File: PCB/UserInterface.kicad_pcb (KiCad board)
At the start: 2 copper layers, 8 parts, among them J10 B2B-PH-K-S, J11 B2B-PH-K-S, J2 Conn_01x12, J3 Conn_01x16, J9 B3B-PH-K-S

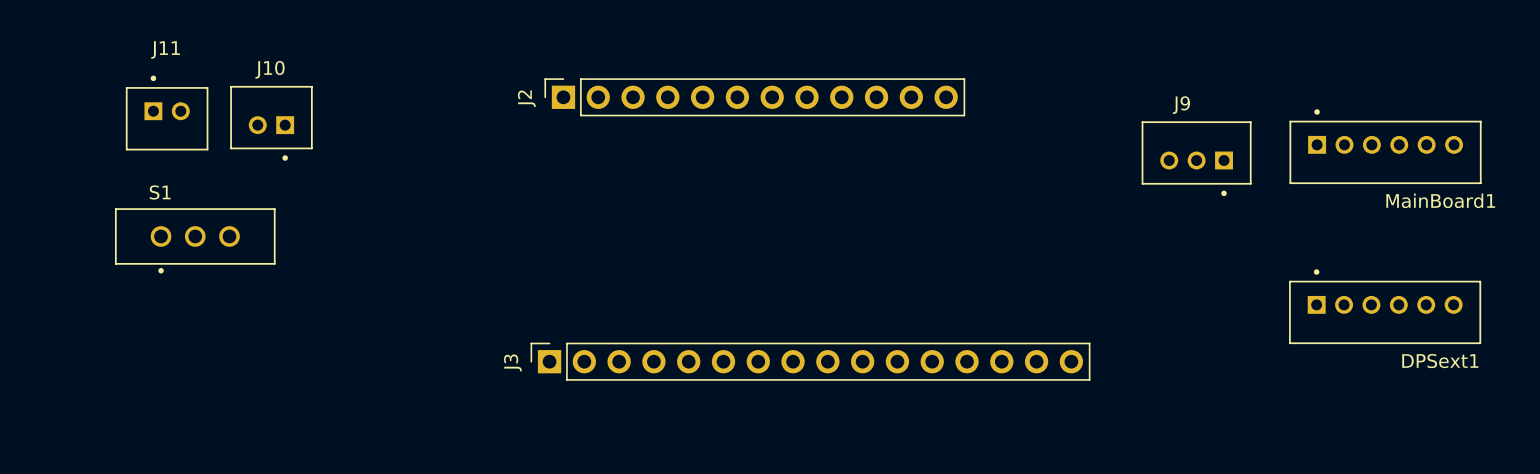
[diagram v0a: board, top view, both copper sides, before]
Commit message: Add files via upload
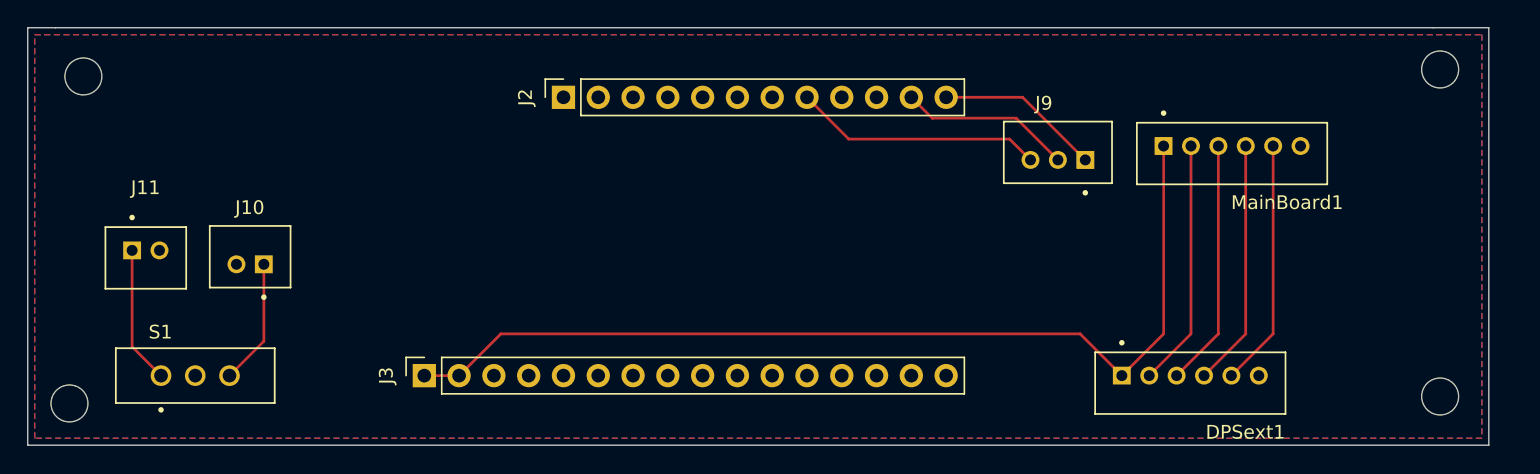
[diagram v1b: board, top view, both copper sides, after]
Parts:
- added REF**: MountingHole_2.7mm_M2.5_ISO7380, MountingHole:MountingHole_2.7mm_M2.5_ISO7380, F.Cu at (73.7, 139.2)
- added REF**: MountingHole_2.7mm_M2.5_ISO7380, MountingHole:MountingHole_2.7mm_M2.5_ISO7380, F.Cu at (173.7, 138.7)
- added REF**: MountingHole_2.7mm_M2.5_ISO7380, MountingHole:MountingHole_2.7mm_M2.5_ISO7380, F.Cu at (173.7, 114.8)
- added REF**: MountingHole_2.7mm_M2.5_ISO7380, MountingHole:MountingHole_2.7mm_M2.5_ISO7380, F.Cu at (74.7, 115.3)
- moved DPSext1 15.1 mm to (155.5, 137.7)
- moved MainBoard1 11.2 mm to (158.5, 120.9)
- moved J10 10.3 mm to (86.9, 128.5)
- moved J11 10.3 mm to (79.2, 128.6)
- moved S1 10.2 mm to (82.8, 137.2)
- moved J9 10.1 mm to (145.8, 120.9)
- moved J3 9.20 mm to (99.6, 137.2)
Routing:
- net /3V3: track 0.00 -> 71.5 mm
- net /OLEDBUTA: track 0.00 -> 18.2 mm
- net /DPSMOSI: track 0.00 -> 18.0 mm
- net /DPSMISO: track 0.00 -> 18.0 mm
- net /DPSCLK: track 0.00 -> 18.0 mm
- net /CS2: track 0.00 -> 18.0 mm
- net /OLEDSCL: track 0.00 -> 12.6 mm
- net /OLEDSDA: track 0.00 -> 12.1 mm
- net Net-(J11-Pad1): track 0.00 -> 10.0 mm
- net Net-(J10-Pad1): track 0.00 -> 9.17 mm
- added copper zone on B.Cu, net GND
- added copper zone on F.Cu, net GND
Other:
- board outline added: 106.7 x 30.5 mm
